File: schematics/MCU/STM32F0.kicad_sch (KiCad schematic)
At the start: 21 parts, among them J2 Conn_ARM_SWD_TagConnect_TC203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, Q1 2N7002, SW13 SW_Push, U1 STM32F072CBTx, Y1 8MHz

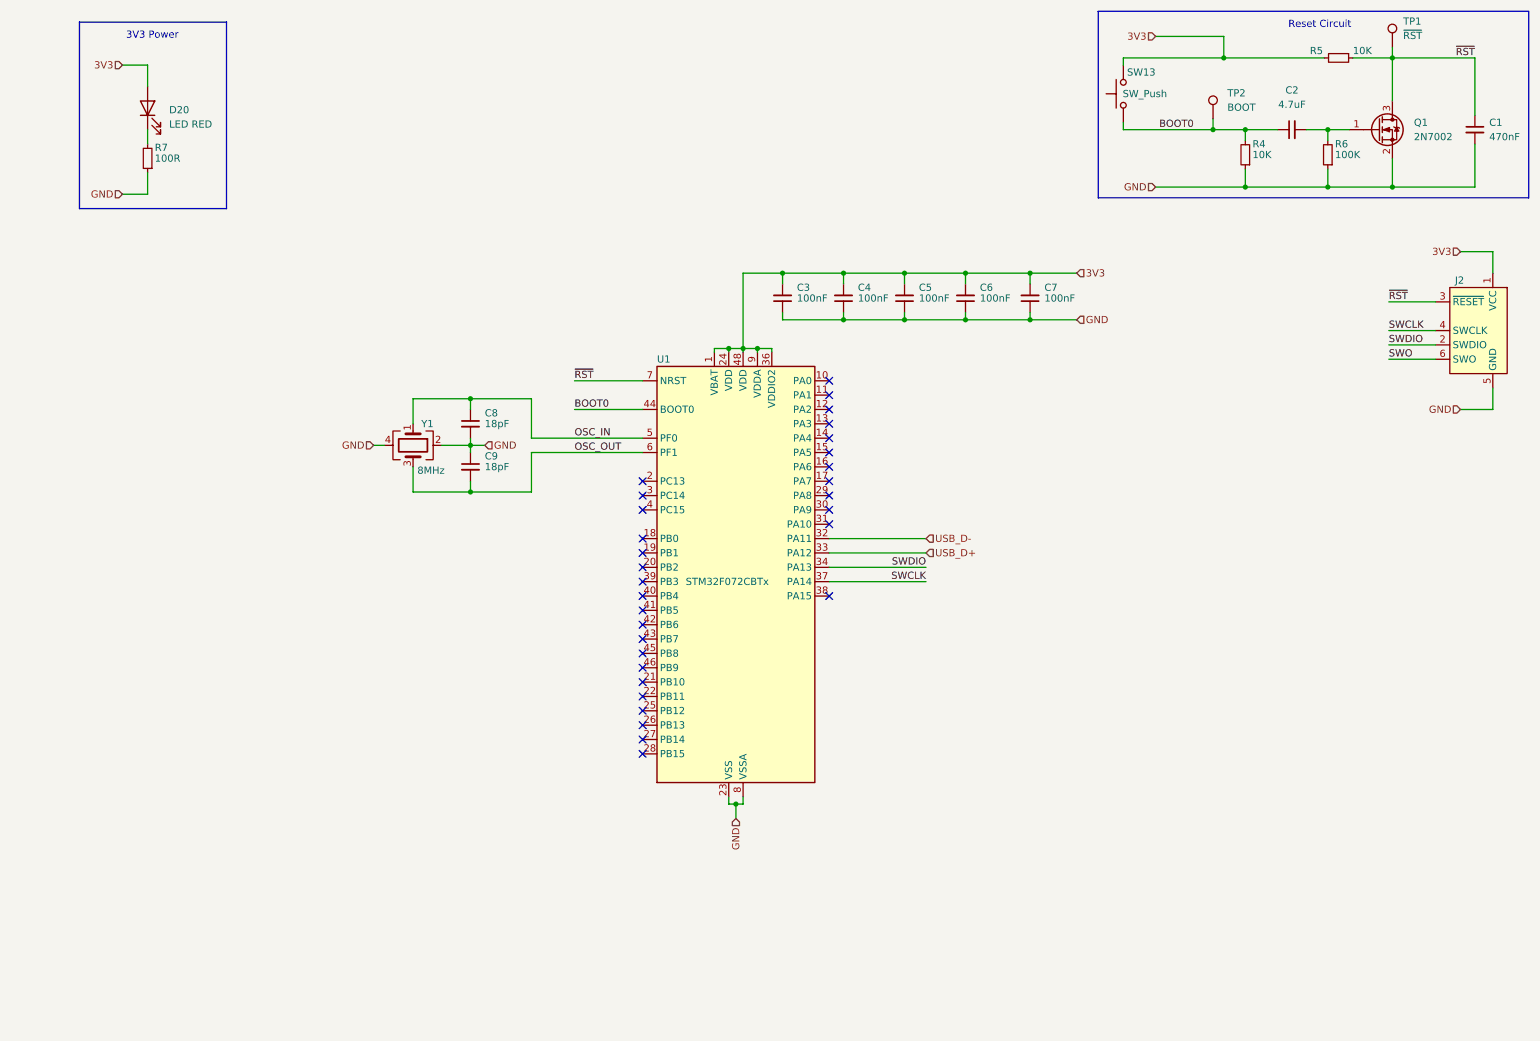
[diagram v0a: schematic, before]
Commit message: Minor updates to STM32, refactor RP2040
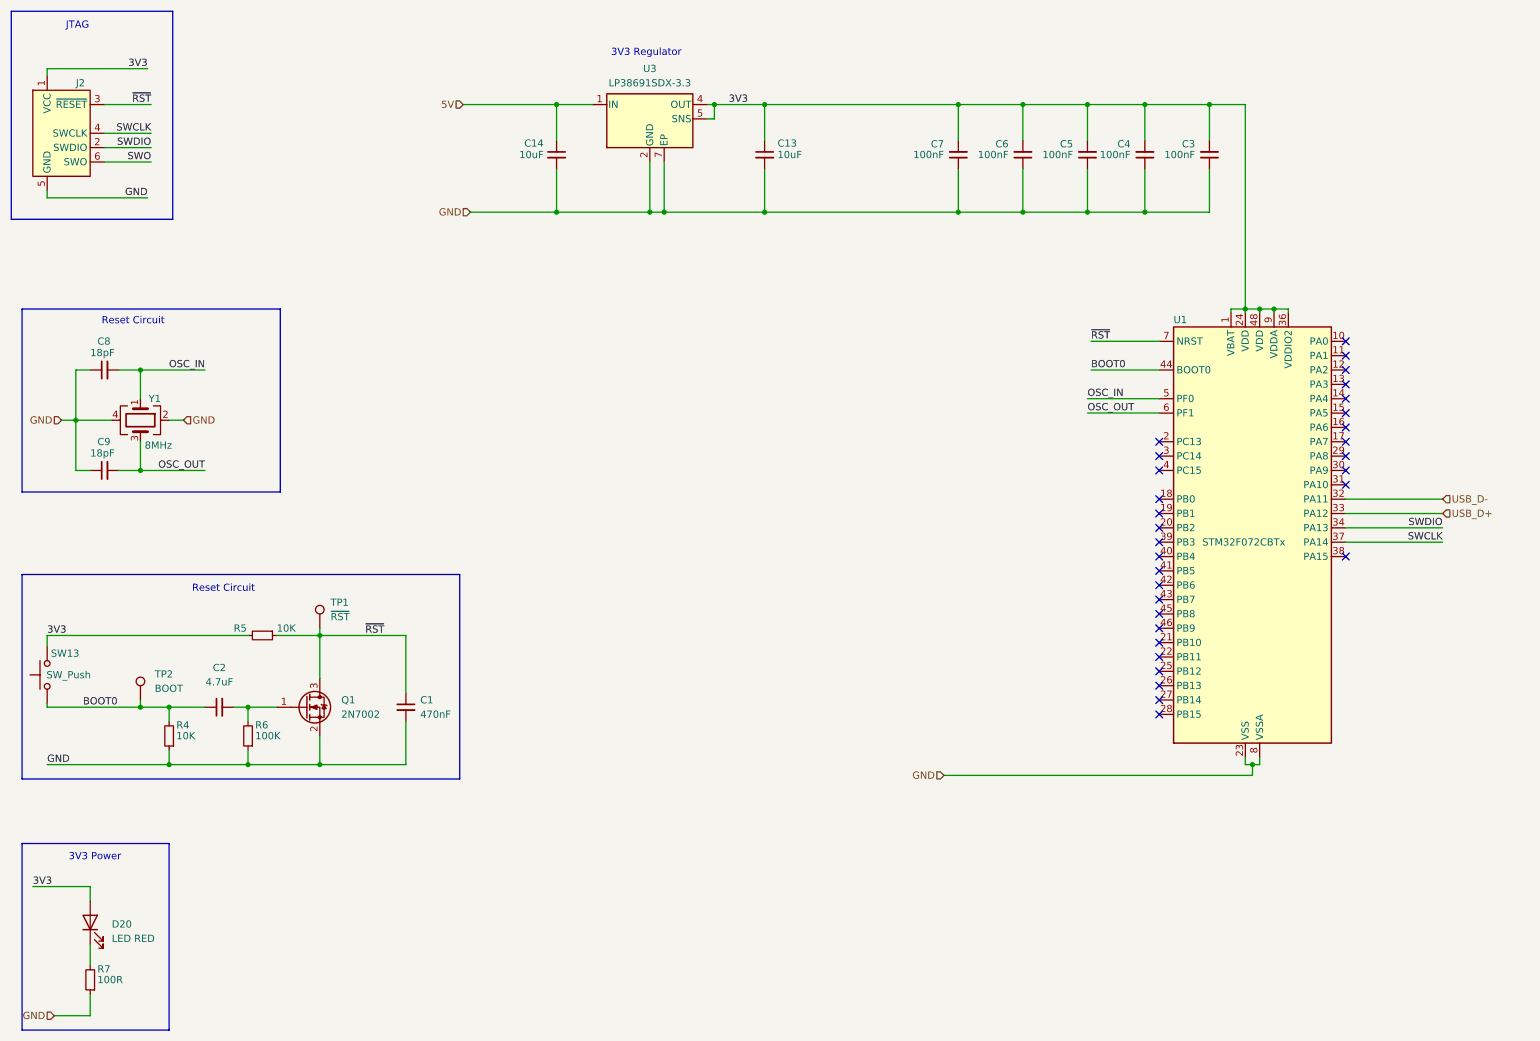
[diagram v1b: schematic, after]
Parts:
- added C13, C14: 10uF, Capacitor_SMD:C_0805_2012Metric, symbol Device:C_Small
- added U3: LP38691SDX-3.3, Package_SON:WSON-6-1EP_3x3mm_P0.95mm, symbol Regulator_Linear:LP38691SD-3.3
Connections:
- net 3V3: now also C13.1, U3.4 (OUT), U3.5 (SNS)
- net GND: now also C8.1, C13.2, C14.2, U3.2 (GND), U3.7 (EP); no longer C8.2
- net OSC_IN: now also C8.2; no longer C8.1
- new net 5V: C14.1, U3.1 (IN), U3.6 (IN)
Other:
- note added: "3V3 Regulator"
- note added: "JTAG"
- moved on the sheet: C1, C2, C3, C4, C5, C6, C7, C9, D20, J2, Q1, R4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
